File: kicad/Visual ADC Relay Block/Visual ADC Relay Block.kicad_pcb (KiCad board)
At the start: 4 copper layers, 33 x 40.6 mm, 30 parts, among them J1 In, J2 Out, K1 DIPxx-1Cxx-51x, Q1 P-NMOS, U1 74HCT595, U2 74HC245

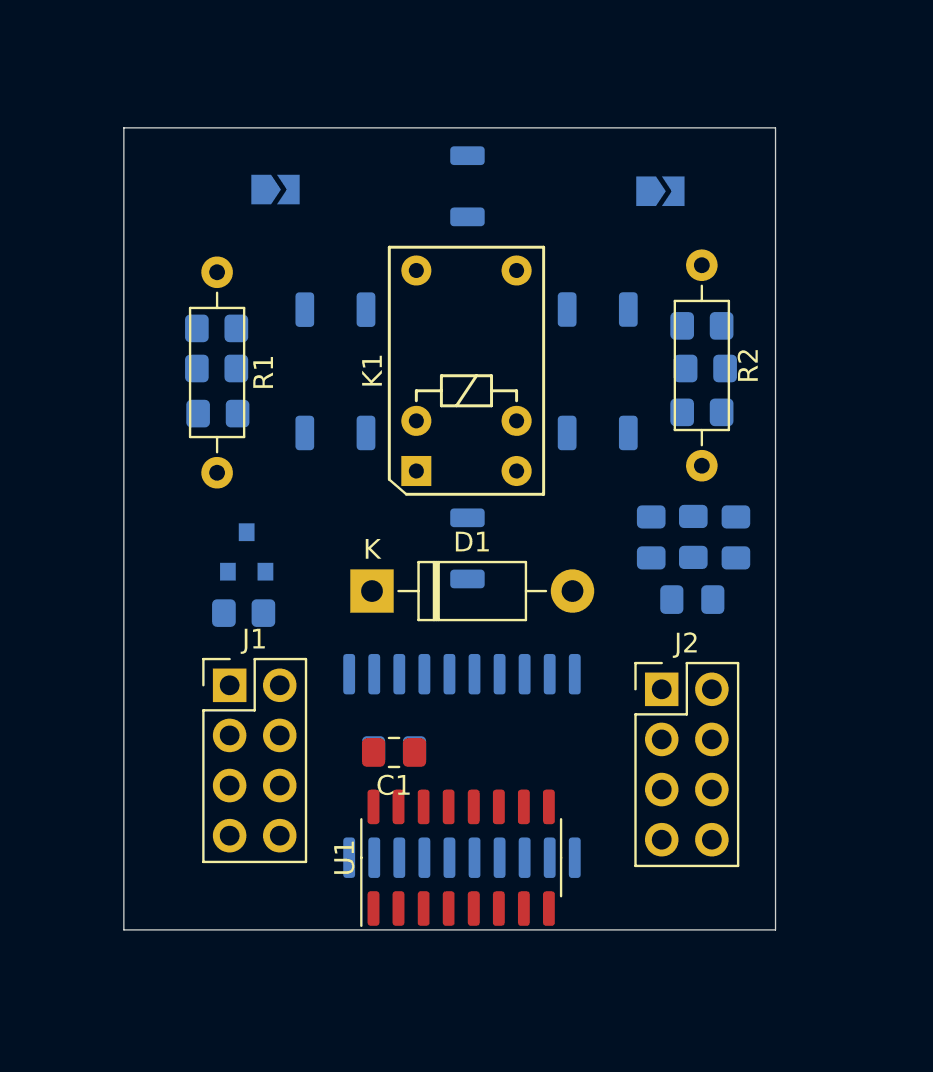
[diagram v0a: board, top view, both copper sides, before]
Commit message: why won't you stop
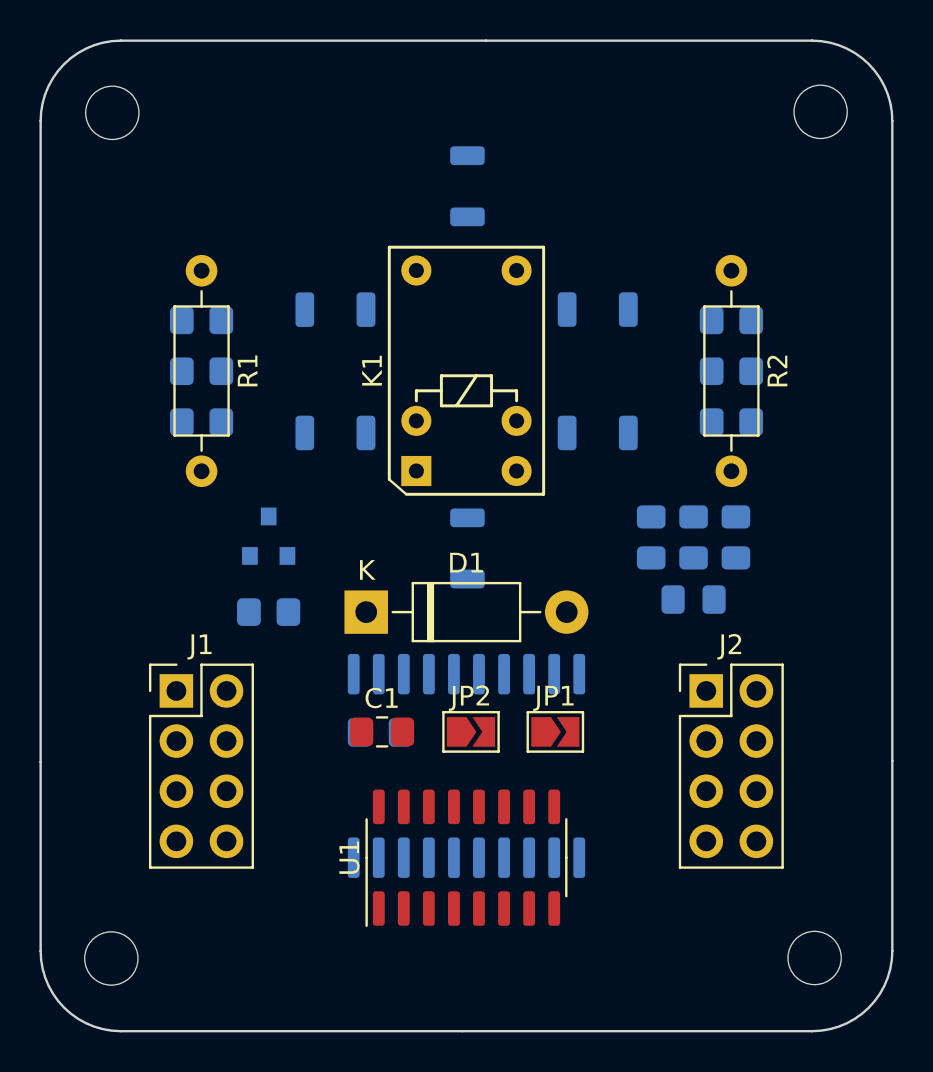
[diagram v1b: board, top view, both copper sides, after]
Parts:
- added H1: MountingHole, MountingHole:MountingHole_2.7mm, F.Cu at (119.4, 86.9)
- added H2: MountingHole, MountingHole:MountingHole_2.7mm, F.Cu at (155.0, 129.7)
- added H3: MountingHole, MountingHole:MountingHole_2.7mm, F.Cu at (155.3, 86.8)
- added H4: MountingHole, MountingHole:MountingHole_2.7mm, F.Cu at (119.4, 129.7)
- JP1, JP2: moved to F.Cu
- moved JP2 29.2 mm to (137.6, 118.2)
- moved JP1 27.9 mm to (141.9, 118.2)
- moved J1 2.71 mm to (122.7, 116.2)
- moved J2 2.26 mm to (149.5, 116.2)
- moved R7 1.57 mm to (150.8, 102.5)
- moved R2 1.52 mm to (150.8, 94.9)
- moved R8 1.52 mm to (150.8, 97.4)
- moved Q1 1.37 mm to (127.4, 108.3)
- moved R6 1.33 mm to (150.8, 100.0)
- moved R3 1.27 mm to (127.4, 112.2)
- moved C1 1.20 mm to (133.1, 118.2), turned to 0 degrees
- moved C2 1.16 mm to (133.0, 118.3)
- moved D1 1.11 mm to (132.3, 112.2)
- moved R5 0.93 mm to (124.0, 102.5), turned to 180 degrees
- moved R9 0.86 mm to (124.0, 97.4)
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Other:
- board size 33 x 40.6 mm -> 43.2 x 50.2 mm
- board text removed: "move diode to inside of relay perimeter"
